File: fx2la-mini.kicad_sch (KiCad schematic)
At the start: 1 part

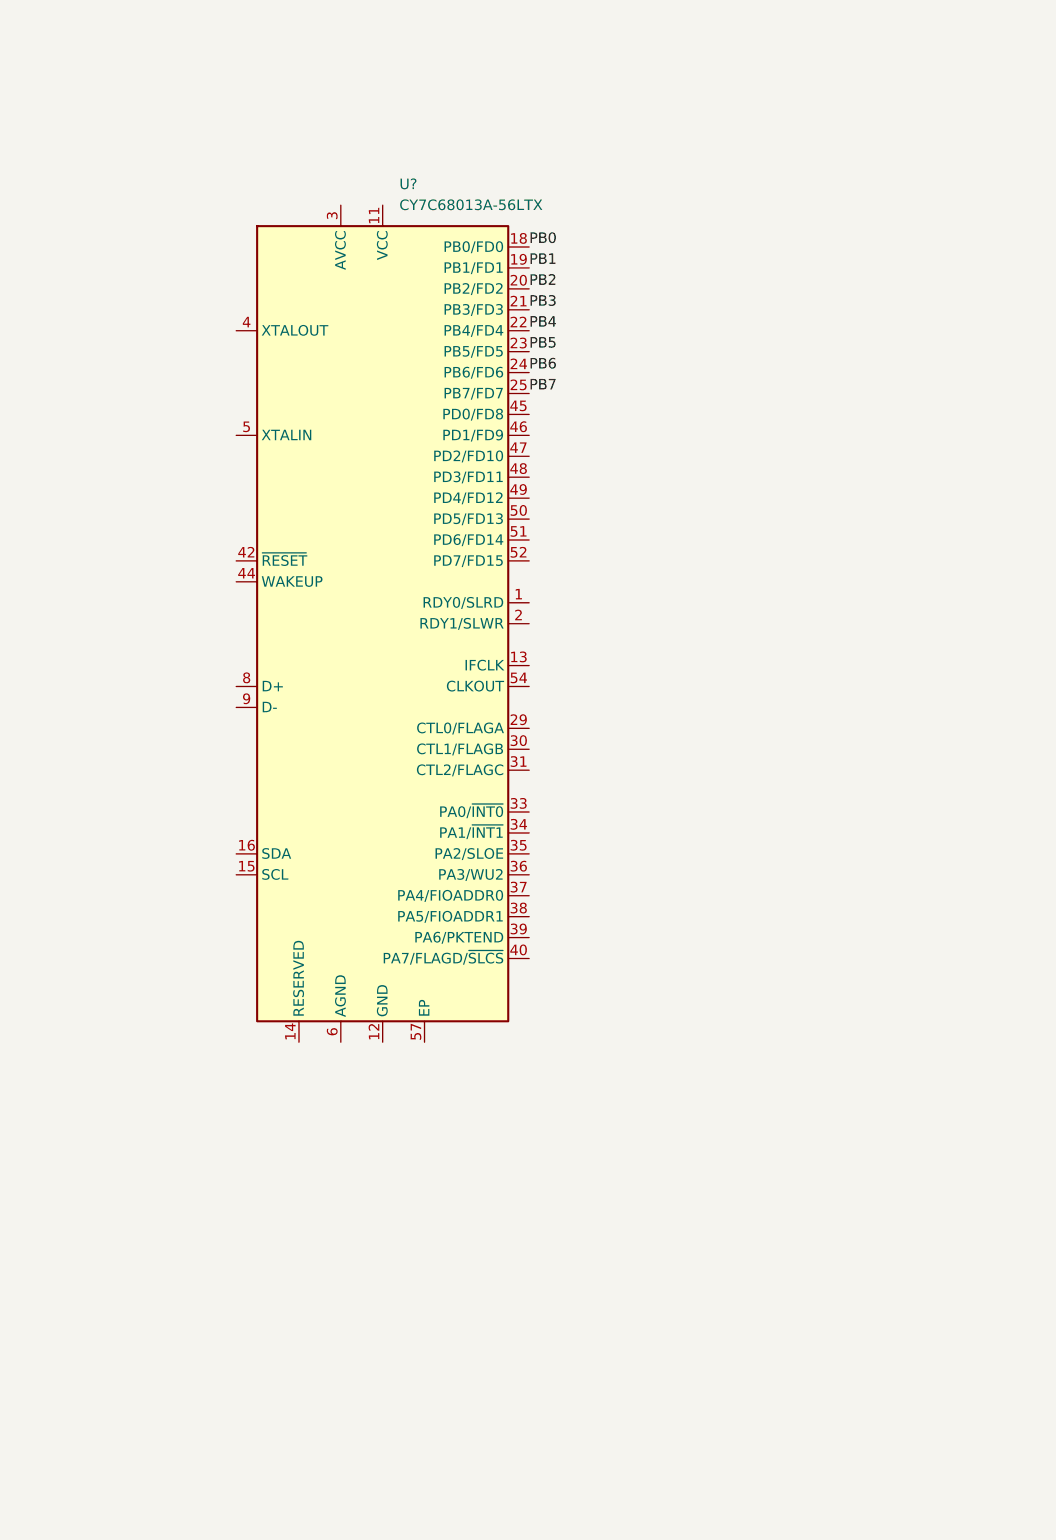
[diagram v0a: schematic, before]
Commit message: Save
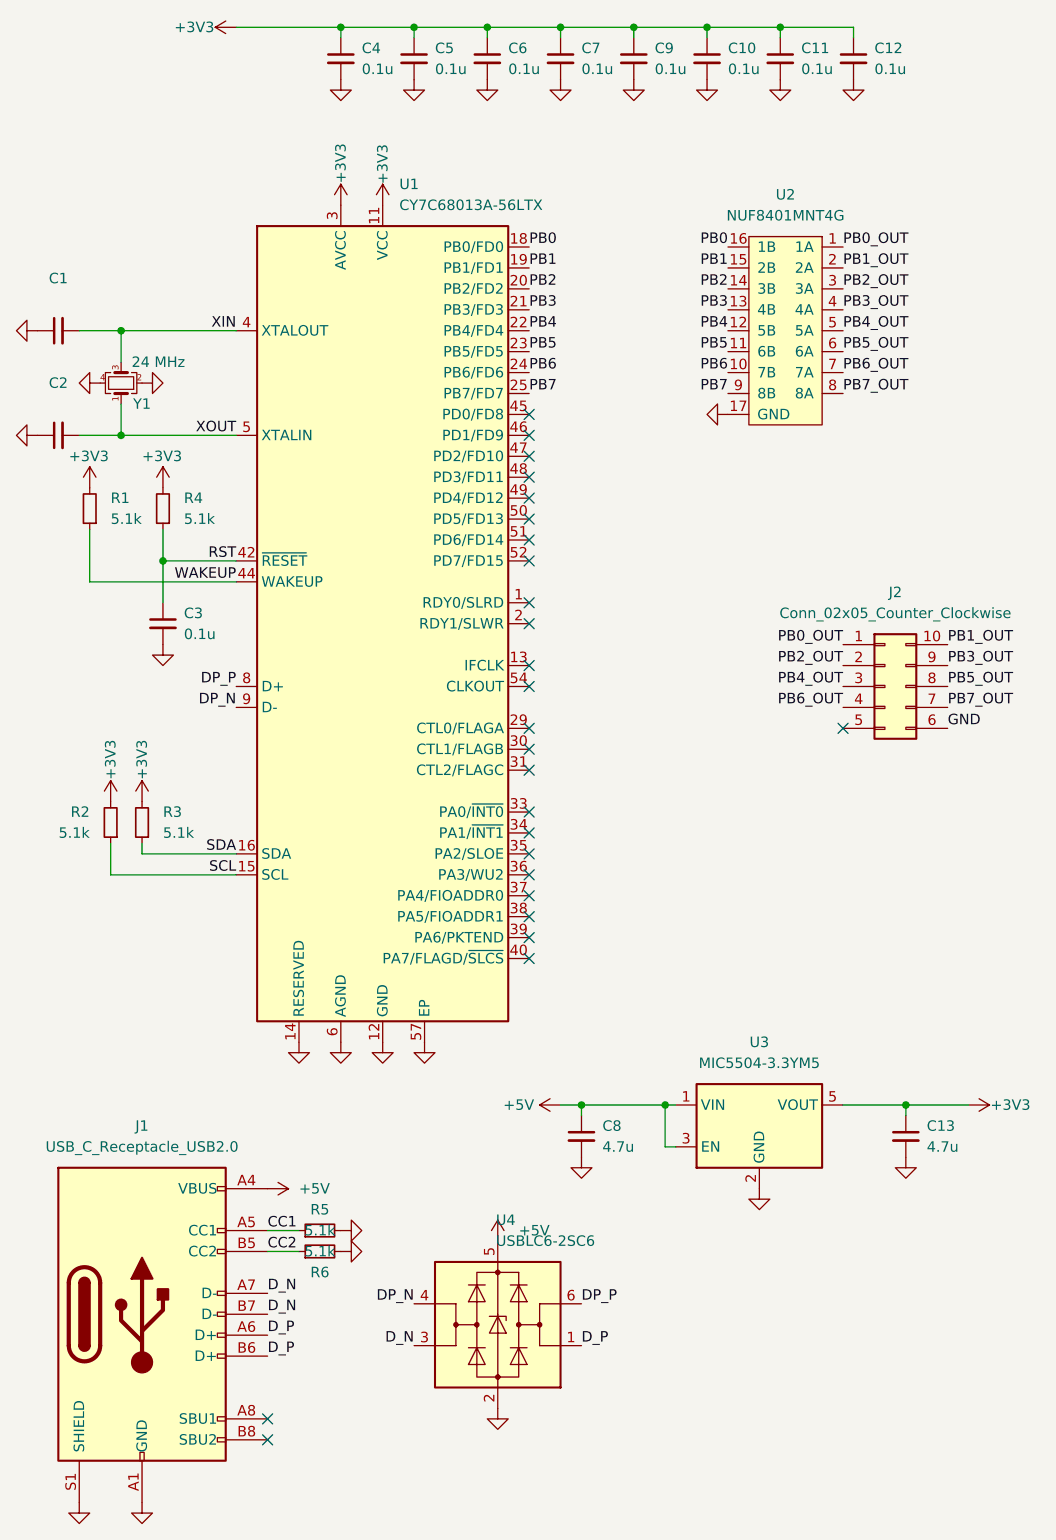
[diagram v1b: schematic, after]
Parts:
- added C1, C2: ~, passive:C_0402, symbol Device:C_Small
- added C10, C11, C12, C3, C4, C5, C6, C7, C9: 0.1u, passive:C_0402, symbol Device:C_Small
- added C13, C8: 4.7u, passive:C_0402, symbol Device:C_Small
- added J1: USB_C_Receptacle_USB2.0, connectors:USB_C_Receptacle_USB4105, symbol Connector:USB_C_Receptacle_USB2.0
- added J2: Conn_02x05_Counter_Clockwise, connectors:2x5_2.54mm_side, symbol Connector_Generic:Conn_02x05_Counter_Clockwise
- added R1, R2, R3, R4, R5, R6: 5.1k, passive:R_0402, symbol Device:R_Small
- added U2: NUF8401MNT4G, dfn:DFN-16-1EP_1.6x4mm_P0.5mm, symbol interface_esd:NUF8401MNT4G
- added U3: MIC5504-3.3YM5, Package_TO_SOT_SMD:SOT-23-5, symbol Regulator_Linear:MIC5504-3.3YM5
- added U4: USBLC6-2SC6, Package_TO_SOT_SMD:SOT-23-6, symbol Power_Protection:USBLC6-2SC6
- added Y1: 24 MHz, crystals:Crystal_4Pin_2.0x1.6mm, symbol Device:Crystal_GND24_Small
- U1: renamed from U?; footprint Package_DFN_QFN:QFN-56-1EP_8x8mm_P0.5mm_EP4.5x5.2mm_ThermalVias_TopTented -> Package_DFN_QFN:QFN-56-1EP_8x8mm_P0.5mm_EP4.5x5.2mm
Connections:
- net PB0: now also U2.16 (1B)
- net PB1: now also U2.15 (2B)
- net PB2: now also U2.14 (3B)
- net PB3: now also U2.13 (4B)
- net PB4: now also U2.12 (5B)
- net PB5: now also U2.11 (6B)
- net PB6: now also U2.10 (7B)
- net PB7: now also U2.9 (8B)
- net GND: now reaches U1.10 (AGND), U1.6 (AGND)
- net GND: now also U1.12 (GND), U1.14 (RESERVED), U1.26 (GND), U1.28 (GND), U1.41 (GND), U1.53 (GND), U1.56 (GND), U1.57 (EP), C1.1, C10.2, C11.2, C12.2, C13.2, C2.1, C3.2, C4.2, C5.2, C6.2, C7.2, C8.2, C9.2, J1.A1 (GND), J1.A12 (GND), J1.B1 (GND), J1.B12 (GND), J1.S1 (SHIELD), J2.6 (Pin_6), R5.2, R6.2, U2.17 (GND), U3.2 (GND), U4.2 (GND), Y1.2, Y1.4
- net +3V3: now reaches U1.11 (VCC), U1.17 (VCC), U1.27 (VCC), U1.32 (VCC), U1.43 (VCC), U1.55 (VCC)
- net +3V3: now also U1.3 (AVCC), U1.7 (AVCC), C10.1, C11.1, C12.1, C13.1, C4.1, C5.1, C6.1, C7.1, C9.1, R1.2, R2.2, R3.2, R4.2, U3.5 (VOUT)
- net SCL: now reaches U1.15 (SCL)
- net SCL: now also R2.1
- net SDA: now reaches U1.16 (SDA)
- net SDA: now also R3.1
- net XIN: now reaches U1.4 (XTALOUT)
- net XIN: now also C1.2, Y1.3
- net RST: now reaches U1.42 (~{RESET})
- net RST: now also C3.1, R4.1
- net WAKEUP: now reaches U1.44 (WAKEUP)
- net WAKEUP: now also R1.1
- net XOUT: now reaches U1.5 (XTALIN)
- net XOUT: now also C2.2, Y1.1
- net DP_P: now reaches U1.8 (D+)
- net DP_P: now also U4.6 (I/O1)
- net DP_N: now reaches U1.9 (D-)
- net DP_N: now also U4.4 (I/O2)
- new net +5V: C8.1, J1.A4 (VBUS), J1.A9 (VBUS), J1.B4 (VBUS), J1.B9 (VBUS), U3.1 (VIN), U3.3 (EN), U4.5 (VBUS)
- new net CC1: J1.A5 (CC1), R5.1
- new net CC2: J1.B5 (CC2), R6.1
- new net D_N: J1.A7 (D-), J1.B7 (D-), U4.3 (I/O2)
- new net D_P: J1.A6 (D+), J1.B6 (D+), U4.1 (I/O1)
- new net PB0_OUT: J2.1 (Pin_1), U2.1 (1A)
- new net PB1_OUT: J2.10 (Pin_10), U2.2 (2A)
- new net PB2_OUT: J2.2 (Pin_2), U2.3 (3A)
- new net PB3_OUT: J2.9 (Pin_9), U2.4 (4A)
- new net PB4_OUT: J2.3 (Pin_3), U2.5 (5A)
- new net PB5_OUT: J2.8 (Pin_8), U2.6 (6A)
- new net PB6_OUT: J2.4 (Pin_4), U2.7 (7A)
- new net PB7_OUT: J2.7 (Pin_7), U2.8 (8A)
- no-connect marks 0 -> 26
